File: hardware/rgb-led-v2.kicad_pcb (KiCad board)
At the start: 2 copper layers, 20 x 25 mm, 26 parts, among them P1 CON-SENSOR2, P2 DEBUG, P3 BOOT, U1 XMC1100, U3 DRILL, U4 DRILL, U5 DRILL, U6 DRILL

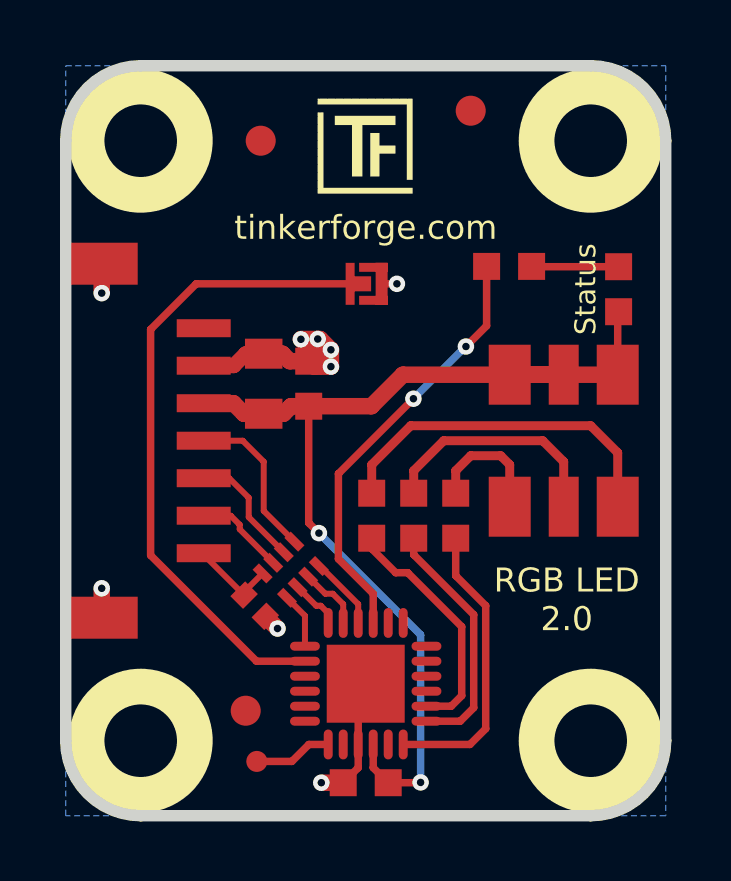
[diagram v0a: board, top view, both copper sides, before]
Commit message: move to new kicad version
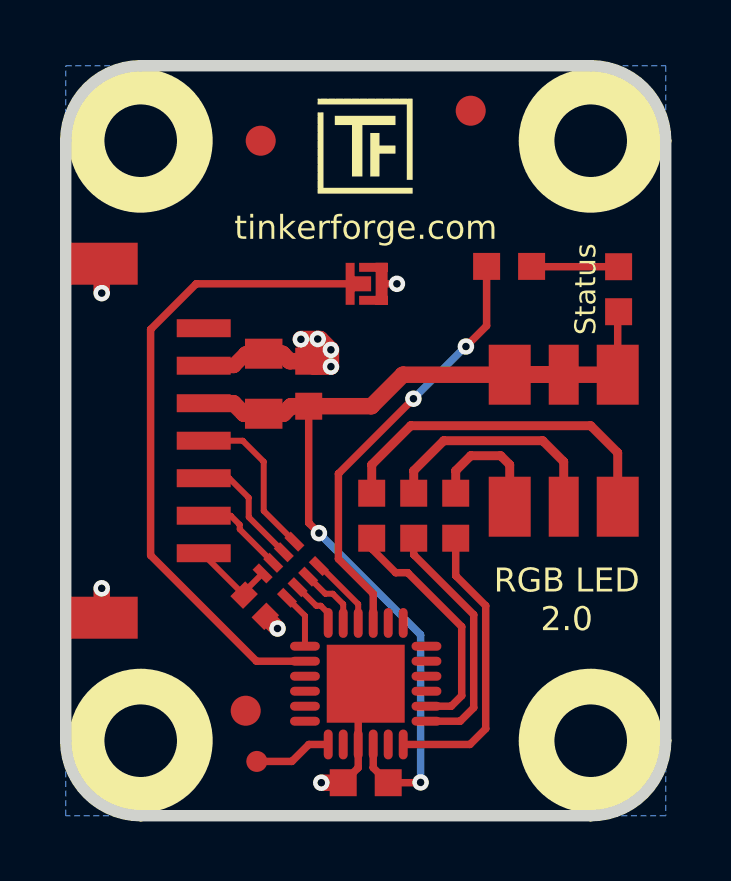
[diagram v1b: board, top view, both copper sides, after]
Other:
- net class Default removed
